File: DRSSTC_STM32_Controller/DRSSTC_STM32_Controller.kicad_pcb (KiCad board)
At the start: 4 copper layers, 100 x 100 mm, 305 parts, among them IC1 UCC27282DR, IC2 UCC27282DR, IC3 UCC27282DR, IC4 UCC27282DR, IC5 SN74LVC14ADR, IC6 SN74LVC11ADR, IC7 SN74LVC11ADR, IC8 PLT237_T10WH, J1 Conn_01x04, J10 Conn_01x04, J11 Conn_01x04, J12 Conn_01x10, J13 USB_C_Receptacle_USB2.0_14P, J14 Conn_01x10, J16 Conn_01x04, J17 Conn_01x10, J2 Conn_01x04, J27 Conn_01x04, J3 Conn_02x05_Odd_Even, J32 Screw_Terminal_01x02, J33 Screw_Terminal_01x02, J4 Screw_Terminal_01x02, J42 Screw_Terminal_01x02, J5 Conn_Coaxial, J6 Conn_Coaxial, J7 Conn_01x04, Q1 QM6006D, Q10 2N7002, Q11 2N7002, Q12 2N7002, Q13 2N7002, Q14 2N7002, Q15 QM6006D, Q16 QM6006D, Q17 QM6006D, Q18 QM6006D, Q19 2N7002, Q2 QM6006D, Q20 2N7002, Q3 QM6006D, Q4 QM6006D, Q5 2N7002, Q6 2N7002, Q7 2N7002, Q8 2N7002, Q9 2N7002, U1 STM32G474RETx, U2 PLR237_T10BK, U3 LF15_TO252, U4 TPS54560BDDA, U7 LV2842XLVDDCR, Y1 Crystal

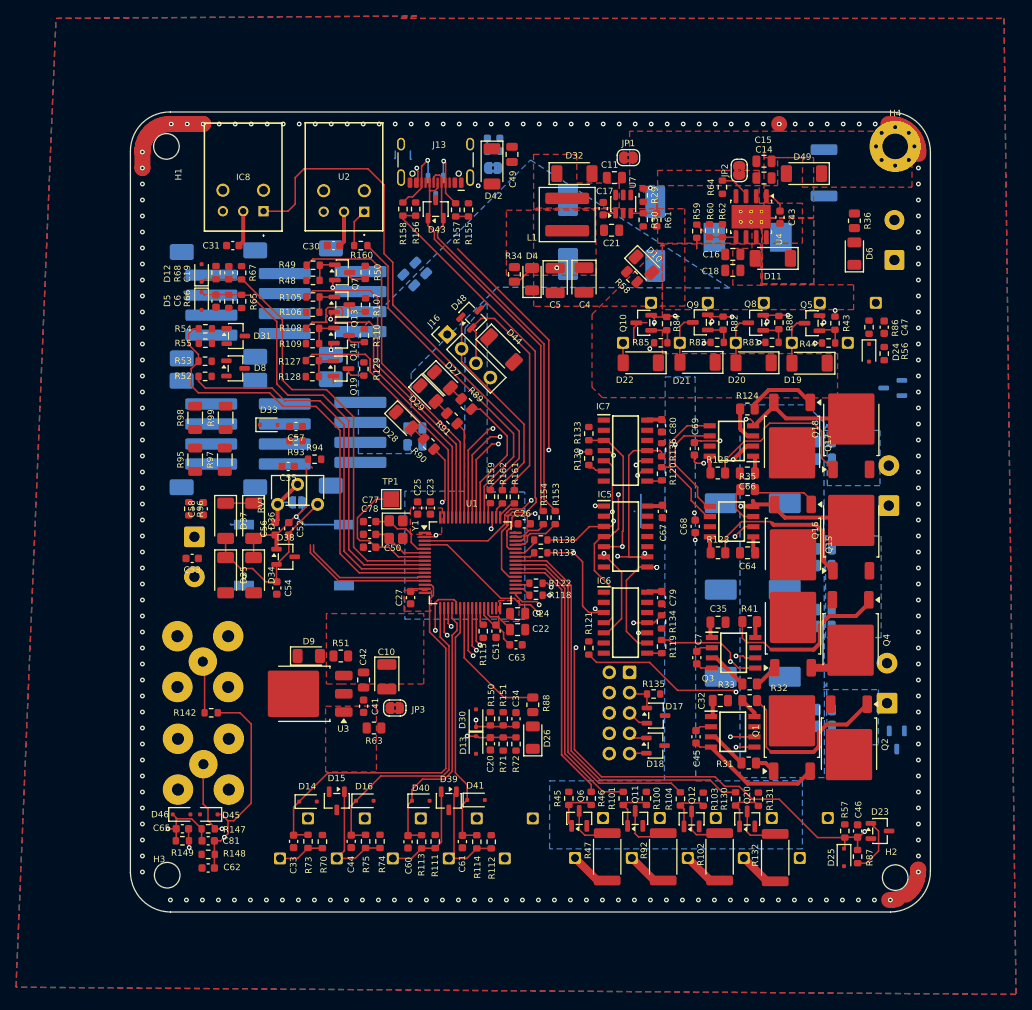
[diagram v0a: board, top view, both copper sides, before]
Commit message: finalize the controller design
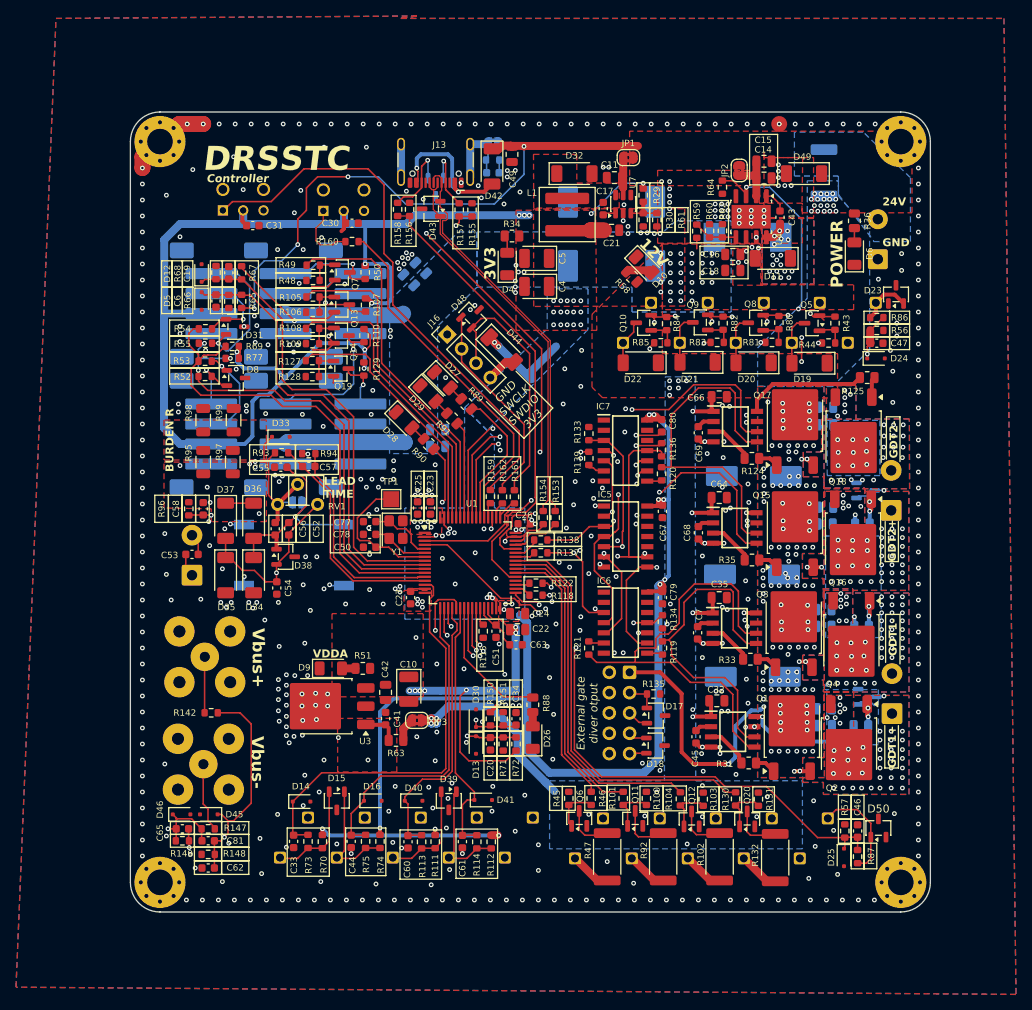
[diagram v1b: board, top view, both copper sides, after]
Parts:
- removed H1, H2, H3: MountingHole, MountingHole:MountingHole_3.2mm_M3
- added D50: ESDA5V3L, Package_TO_SOT_SMD:SOT-23-3, F.Cu at (322.6, 152.0)
- added G***: LOGO, LOGO, B.Cu at (292.3, 119.6)
- added G***: LOGO, LOGO, B.Cu at (292.3, 105.8)
- added H5: MountingHole_Pad, MountingHole:MountingHole_3.2mm_M3_Pad_Via, F.Cu at (325.4, 158.8)
- added H6: MountingHole_Pad, MountingHole:MountingHole_3.2mm_M3_Pad_Via, F.Cu at (232.8, 66.2)
- added H7: MountingHole_Pad, MountingHole:MountingHole_3.2mm_M3_Pad_Via, F.Cu at (232.8, 158.8)
- added R69: 4k7, Resistor_SMD:R_0603_1608Metric, F.Cu at (241.8, 91.8)
- added R77: 4k7, Resistor_SMD:R_0603_1608Metric, F.Cu at (241.8, 93.3)
- IC8, R123, R32, R41, U2: moved to B.Cu
- moved D23 67.1 mm to (324.8, 85.3), turned to 90 degrees
- moved R125 22.2 mm to (321.2, 95.7)
- moved R123 18.4 mm to (320.6, 114.0)
- moved R32 14.3 mm to (320.4, 139.2)
- moved R41 14.0 mm to (320.5, 126.8), turned to 0 degrees
- moved D3 13.2 mm to (321.0, 109.8), turned to 0 degrees
- moved C66 10.2 mm to (302.7, 98.1), turned to 0 degrees
- moved R35 8.82 mm to (306.8, 118.5)
- moved C64 7.76 mm to (302.7, 110.7), turned to 0 degrees
- moved D2 6.55 mm to (321.2, 135.6), turned to 0 degrees
- moved R124 6.20 mm to (306.8, 105.8)
- moved C4 5.95 mm to (279.9, 84.3), turned to 180 degrees
- moved C57 5.25 mm to (251.4, 106.8), turned to 0 degrees
- moved C29 5.20 mm to (315.9, 114.0)
- moved C37 5.20 mm to (316.0, 111.9)
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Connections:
- net Net-(U1-PA11) renamed /MCU and comms/USB_N
- net Net-(U1-PA12) renamed /MCU and comms/USB_P
- D23 pad 1: /MCU and comms/GPIO_2 -> unconnected-(D23-K-Pad1)
- IC6 pad 1: unconnected-(IC6-1A-Pad1) -> GND
- IC6 pad 13: unconnected-(IC6-1C-Pad13) -> GND
- IC6 pad 2: unconnected-(IC6-1B-Pad2) -> GND
- IC7 pad 1: unconnected-(IC7-1A-Pad1) -> GND
- IC7 pad 13: unconnected-(IC7-1C-Pad13) -> GND
- IC7 pad 2: unconnected-(IC7-1B-Pad2) -> GND
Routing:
- net GND: track 397.8 -> 817.7 mm, vias 194 -> 577
- net +3V3: track 16.2 -> 335.5 mm, vias 2 -> 54
- net +24V: track 0.54 -> 104.3 mm, vias 0 -> 127
- net +12V: track 9.85 -> 87.4 mm, vias 0 -> 45
- net VDDA: track 4.26 -> 42.0 mm, vias 0 -> 7
- net Net-(IC3-HI): track 27.6 -> 63.2 mm, vias 2 -> 3
- net /MCU and comms/12V_EN: track 57.8 -> 84.6 mm, vias 1 -> 5
- net /MCU and comms/GPIO1: track 47.0 -> 72.9 mm, vias 1 -> 2
- net Net-(IC3-LI): track 18.4 -> 42.5 mm
- net Net-(Q18-G): track 22.0 -> 2.58 mm
- net Net-(IC1-HI): track 36.6 -> 55.7 mm, vias 3 -> 0
- net Net-(Q2-G): track 22.7 -> 3.84 mm, vias 0 -> 2
- net Net-(J27-Pin_4): track 0.00 -> 18.6 mm, vias 0 -> 1
- net Net-(Q4-G): track 22.6 -> 4.44 mm, vias 0 -> 2
- net Net-(D35-K): track 21.9 -> 38.5 mm, vias 0 -> 3
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- added copper zone on B.Cu, net /GDT_driver/GDT1+
- added copper zone on F.Cu, net /GDT_driver/GDT1+
- added copper zone on B.Cu, net /GDT_driver/GDT1-
- added copper zone on F.Cu, net /GDT_driver/GDT1-
- added copper zone on B.Cu, net /GDT_driver/GDT2+
- added copper zone on F.Cu, net /GDT_driver/GDT2+
- added copper zone on B.Cu, net /GDT_driver/GDT2-
- added copper zone on F.Cu, net /GDT_driver/GDT2-
- added copper zone on B.Cu, net /PSU/24Vin
- added copper zone on F.Cu, net Net-(D33-K)
- added copper zone on F.Cu, net Net-(R95-Pad2)
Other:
- outline, holes or cut-outs redrawn
- board text added: "-"
- board text added: "07.2026 J.Soszynski"
- board text added: "12V"
- board text added: "24V"
- board text added: "3V3"
- board text added: "BURDEN R"
- board text added: "CT+"
- board text added: "CT-"
- board text added: "Connenct external DC-blocking caps if necesary !!!"
- board text added: "Controller"
- board text added: "DRSSTC"
- board text added: "DRSSTC Controller"
- board text added: "External gate diver otput"
- board text added: "External series resistace needed !!!"
- board text added: "FAN1"
- board text added: "FAN2"
- board text added: "FAN3"
- board text added: "FAN4"
- board text added: "FUSE"
- board text added: "G1+"
- board text added: "G1-"
- board text added: "G2+"
- board text added: "G2-"
- board text added: "GDT1+"
- board text added: "GDT1-"
- board text added: "GDT2+"
- board text added: "GDT2-"
- board text added: "GND"
- board text added: "GND SWCLK SWDIO 3V3"
- board text added: "GPIO1"
- board text added: "GPIO2"
- board text added: "Github"
- board text added: "I2C"
- board text added: "LEAD TIME"
- board text added: "LED1"
- board text added: "LED2"
- board text added: "LED3"
- board text added: "LED4"
- board text added: "NTC1"
- board text added: "NTC2"
- board text added: "NTC3"
- board text added: "NTC4"
- board text added: "POWER"
- board text added: "PWM"
- board text added: "REV. 1.0"
- board text added: "REl1"
- board text added: "REl2"
- board text added: "REl3"
- board text added: "REl4"
- board text added: "RXD"
- board text added: "SDA"
- board text added: "SLC"
- board text added: "Solder GDTs directly"
- board text added: "Solder directly"
- board text added: "TXD"
- board text added: "VDDA"
- board text added: "Vbus+"
- board text added: "Vbus-"
